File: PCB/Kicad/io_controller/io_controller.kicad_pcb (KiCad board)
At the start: 6 copper layers, 149.2 x 100 mm, 128 parts, among them J1 Conn_02x10_Odd_Even, J2 Conn_02x10_Odd_Even, J4 Conn_01x04, SW1 SW_DIP_x04

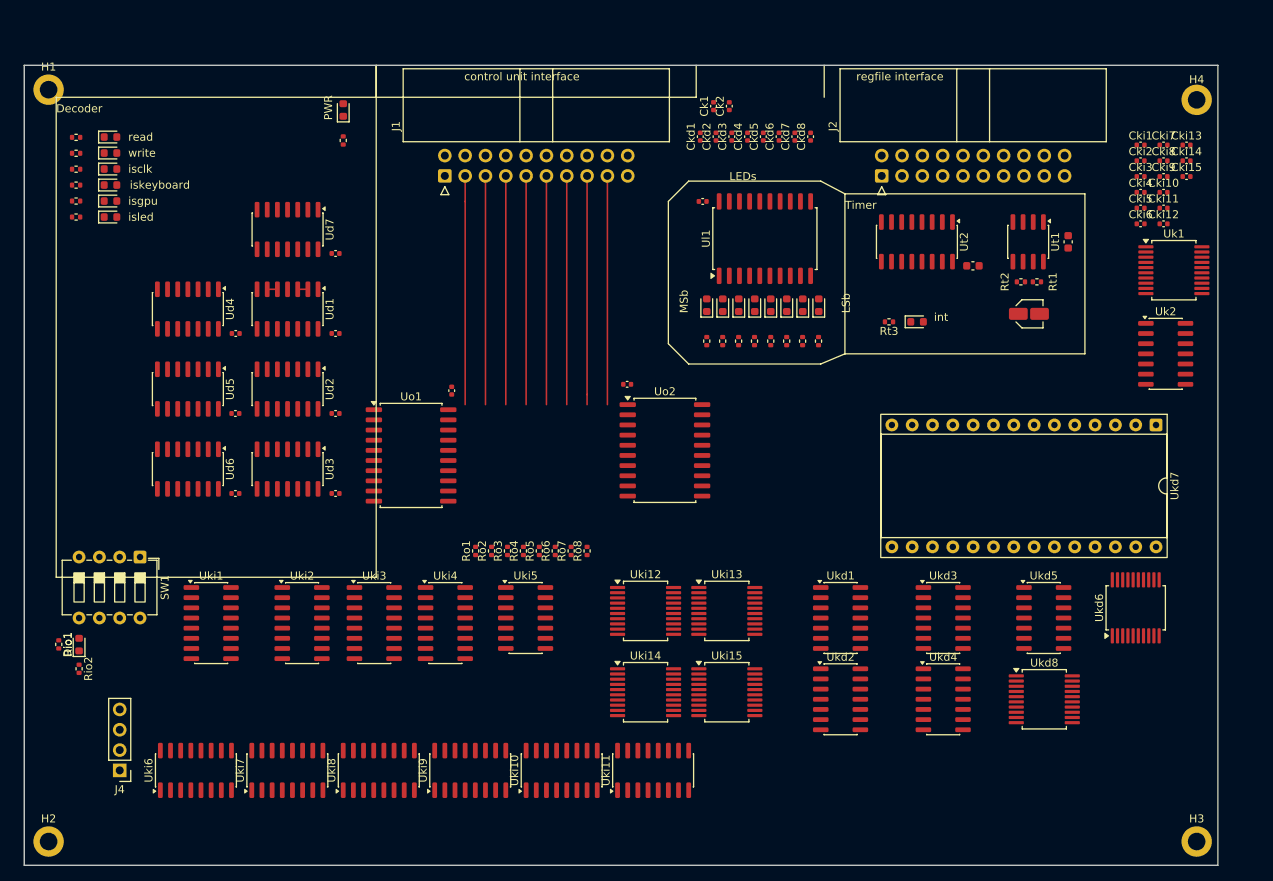
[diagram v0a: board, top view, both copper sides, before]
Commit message: io controller update
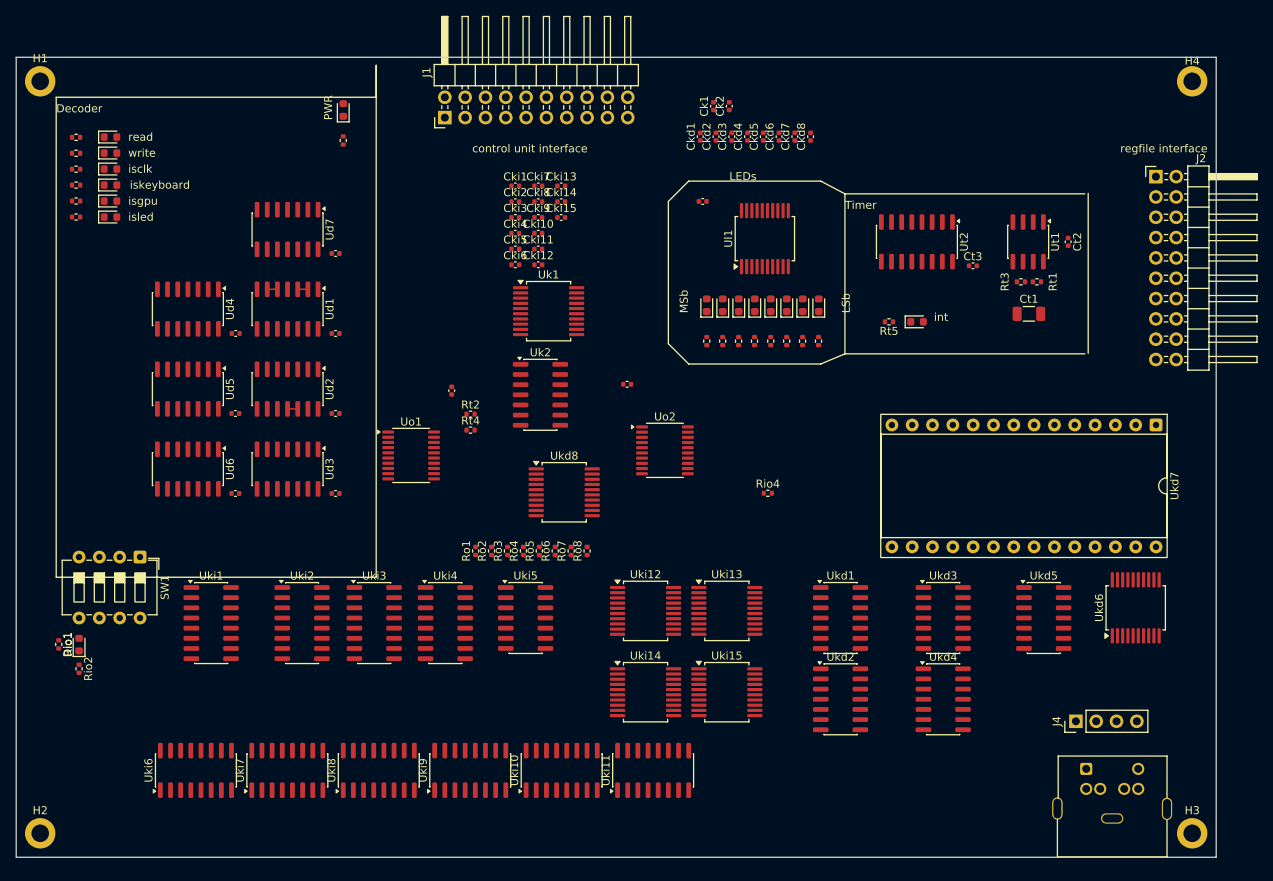
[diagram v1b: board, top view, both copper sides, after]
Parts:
- added J3: Mini-DIN-6, mALUch_lib:MiniDin6_PS2, F.Cu at (148.8, 104.0)
- added Rio4: 10k, Resistor_SMD:R_0402_1005Metric, F.Cu at (109.0, 69.5)
- added Rt2: 10k, Resistor_SMD:R_0402_1005Metric, F.Cu at (71.8, 59.6)
- added Rt4: 10k, Resistor_SMD:R_0402_1005Metric, F.Cu at (71.8, 61.6)
- C1, Cd1, Cd2, Cd3, Cd4, Cd5, Cd6, Cd7, Ck1, Ck2, Ckd1, Ckd2, Ckd3, Ckd4, Ckd5, Ckd6, Ckd7, Ckd8, Cki1, Cki10, Cki11, Cki12, Cki13, Cki14, Cki15, Cki2, Cki3, Cki4, Cki5, Cki6, Cki7, Cki8, Cki9, Co1, Co2: value 0.1u -> 100nF
- Ct1: value 33n -> 33u; footprint Capacitor_SMD:C_Elec_3x5.4 -> Capacitor_SMD:C_1206_3216Metric
- Ct2, Ct3: value 0.1u -> 100nF; footprint Capacitor_SMD:C_0603_1608Metric -> Capacitor_SMD:C_0402_1005Metric
- Dio1: value green -> yellow
- Dl1, Dl2, Dl3, Dl4, Dl5, Dl6, Dl7, Dl8: value red -> blue
- J1, J2: footprint Connector_IDC:IDC-Header_2x10_P2.54mm_Horizontal -> mALUch_lib:PinHeader_2x10_P2.54mm_Horizontal
- Rd1, Rd2, Rd3, Rd4, Rd5, Rd6: value 470 -> 680
- Rt1: value 4.7k -> 10k
- Rt3: renamed from Rt2; value 22k -> 10k
- Ud1, Ud2, Ud3, Uk2, Ukd4, Ukd5: value 74LS02 -> 7402
- Ud4, Ud5, Ud6, Ud7, Ukd1, Ukd2, Ukd3, Uki5: value 74LS08 -> 7408; footprint Package_SO:SOIC-14_3.9x8.7mm_P1.27mm -> Package_SO:SO-14_3.9x8.65mm_P1.27mm
- Uk1, Ukd6, Ukd8, Uki12, Uki13, Uki14, Uki15: value 74LS377 -> 74377
- Uki1, Uki10, Uki11, Uki2, Uki3, Uki4, Uki6, Uki7, Uki8, Uki9, Ut2: value 74LS195 -> 74195
- Ul1: value 74LS377 -> 74377; footprint Package_SO:SOIC-20W_7.5x12.8mm_P1.27mm -> Package_SO:SSOP-20_5.3x7.2mm_P0.65mm
- Uo1, Uo2: value 74LS245 -> 74245; footprint Package_SO:SOIC-20W_7.5x12.8mm_P1.27mm -> Package_SO:TSSOP-20_4.4x6.5mm_P0.65mm
- moved J4 119.7 mm to (147.5, 98.0), turned to 90 degrees
- moved Cki1 78.3 mm to (77.4, 31.1)
- moved Cki2 78.3 mm to (77.4, 33.1)
- moved Cki3 78.3 mm to (77.4, 35.0)
- moved Cki4 78.3 mm to (77.4, 37.0)
- moved Cki5 78.3 mm to (77.4, 39.0)
- moved Cki6 78.3 mm to (77.4, 40.9)
- moved Uk1 78.3 mm to (81.5, 46.7)
- moved Cki13 78.3 mm to (83.1, 31.1)
- moved Cki14 78.3 mm to (83.1, 33.1)
- moved Cki15 78.3 mm to (83.1, 35.0)
- moved Uk2 78.3 mm to (80.5, 57.2)
- moved Cki10 78.3 mm to (80.3, 37.0)
- moved Cki11 78.3 mm to (80.3, 39.0)
- moved Cki12 78.3 mm to (80.3, 40.9)
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- renumbered Rt3 to Rt5
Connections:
- net /key_read renamed /decoder/key_read
- net /timer_clk_en renamed /decoder/timerclk_en
- net /~{led_clk_en} renamed /LEDs/~{clk_en}
- net /~{out_gpu} renamed /decoder/~{gpu_out}
- net /~{out_key} renamed /decoder/~{key_out}
- net /~{timer_read} renamed /decoder/~{timer_read}
- Rt3 pad 1: Net-(Ut1-THR) -> Net-(Rt3-Pad1)
- SW1 pad 2: Net-(SW1-Pad2) -> GND
- SW1 pad 3: Net-(SW1-Pad2) -> GND
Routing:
- net /iobus7: track 28.6 -> 0.00 mm
- net /iobus6: track 28.6 -> 0.00 mm
- net /iobus5: track 28.6 -> 0.00 mm
- net /iobus4: track 28.6 -> 0.00 mm
- net /iobus3: track 28.6 -> 0.00 mm
- net /iobus2: track 28.6 -> 0.00 mm
- net /iobus1: track 28.6 -> 0.00 mm
- net /iobus0: track 28.6 -> 0.00 mm
- net Net-(Ud2-Pad11): track 0.00 -> 1.27 mm
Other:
- board size 149.2 x 100 mm -> 150 x 100 mm
